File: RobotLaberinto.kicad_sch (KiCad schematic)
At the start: 33 parts, among them J1 VL53LDK, J2 VL53LDK, J3 VL53LDK, J4 VL53LDK, J5 VL53LDK, J6 BNO08, U1 DRV8833PWP, U2 ESP32-C3_SUPERMINI_TH, U3 MP2307, U4 CNY70

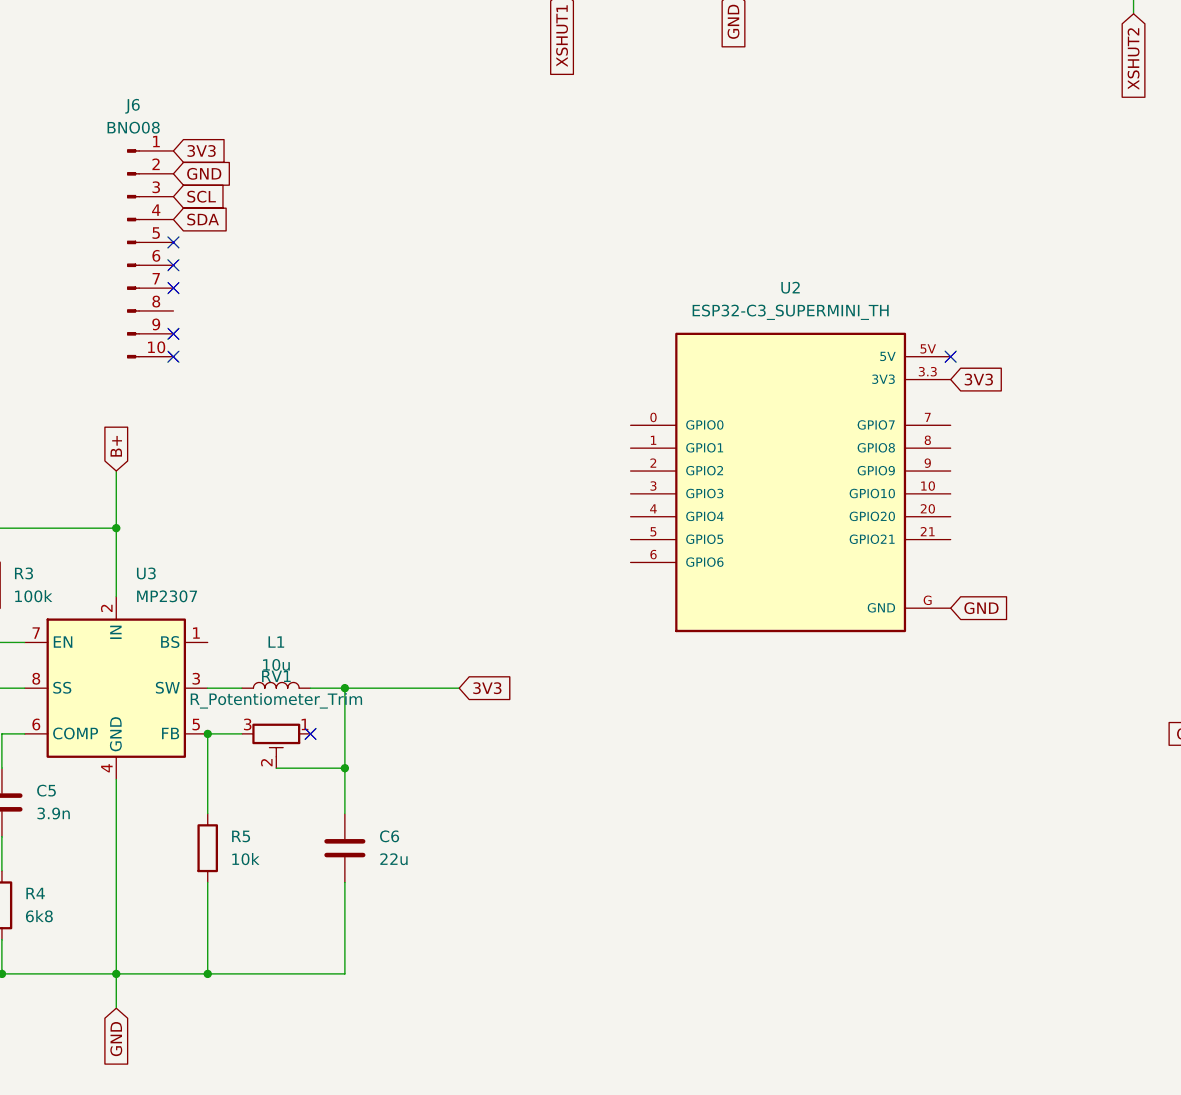
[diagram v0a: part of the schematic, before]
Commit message: trazado
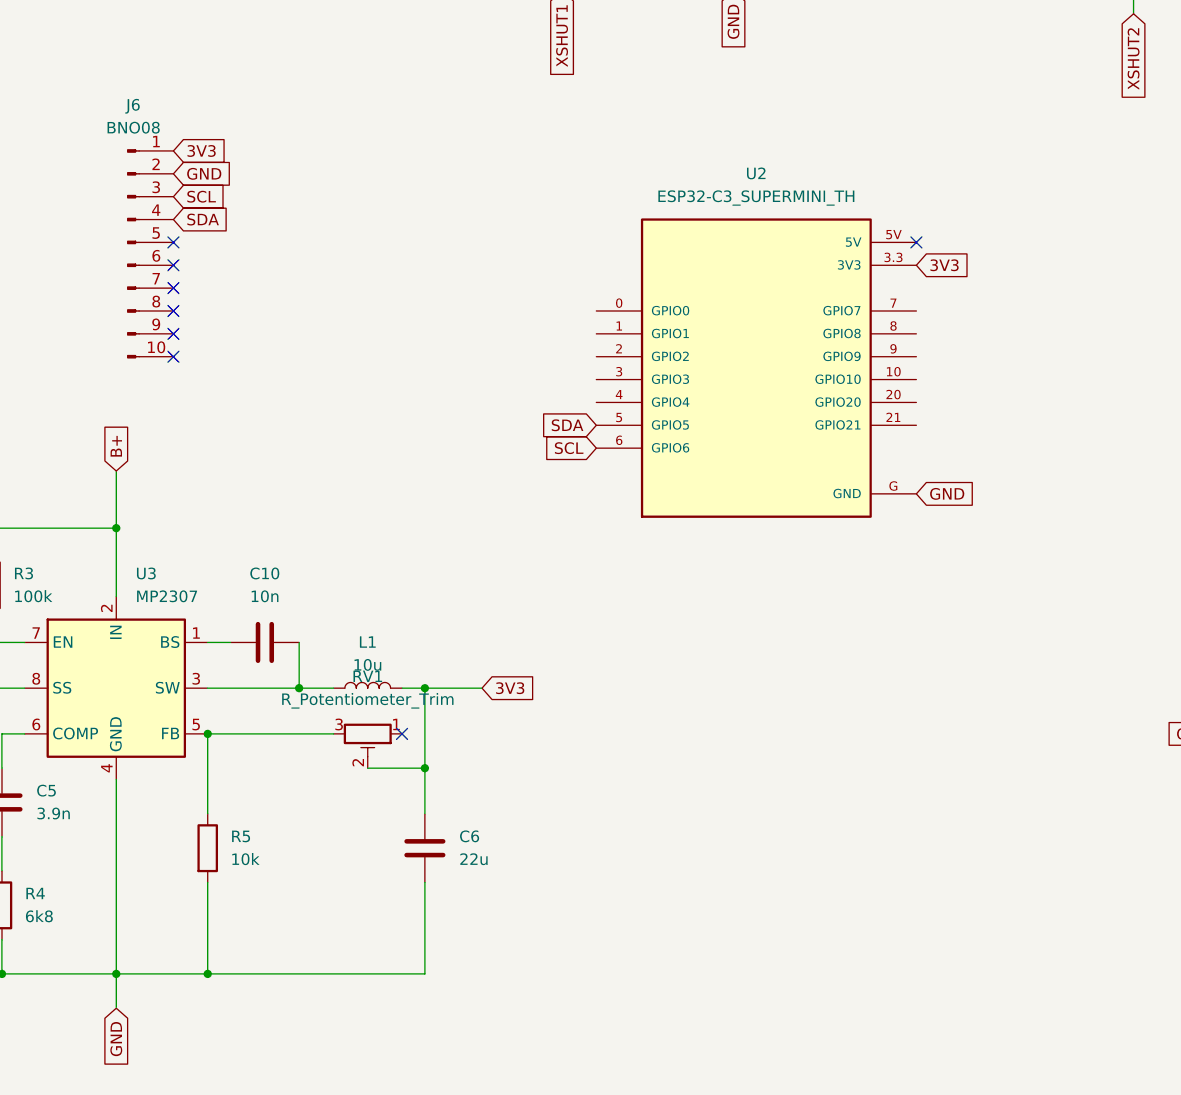
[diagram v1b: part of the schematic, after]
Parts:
- added C10: 10n, Capacitor_SMD:C_0805_2012Metric_Pad1.18x1.45mm_HandSolder, symbol Device:C
- C1: footprint (none) -> Capacitor_SMD:C_0805_2012Metric_Pad1.18x1.45mm_HandSolder
- C3, C6: footprint Capacitor_SMD:C_0805_2012Metric_Pad1.18x1.45mm_HandSolder -> (none)
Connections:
- net SCL: now also U2.6 (GPIO6)
- net SDA: now also U2.5 (GPIO5)
- net at L1.1, U3.3 (SW): now also C10.1
- net at U3.1 (BS): now also C10.2
- no-connect marks 8 -> 9
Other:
- moved on the sheet: C6, L1, RV1, U2
